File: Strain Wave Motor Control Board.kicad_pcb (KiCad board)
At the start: 2 copper layers, 72 parts, among them J1 GSB1C41110SSHR, J2 S4B-XH-SM4-TB, Q1 CSD18531Q5A, Q2 AO4407A, Q3 CSD18531Q5A, Q4 AO4407A, Q5 SI4178DY-T1-GE3, Q6 AO4407A, U1 HUSB238A-xxxxx-QN16R, U2 BQ7791500PWR, U3 LTC4007, U4 LM2596S-5, U5 ESP32-C6

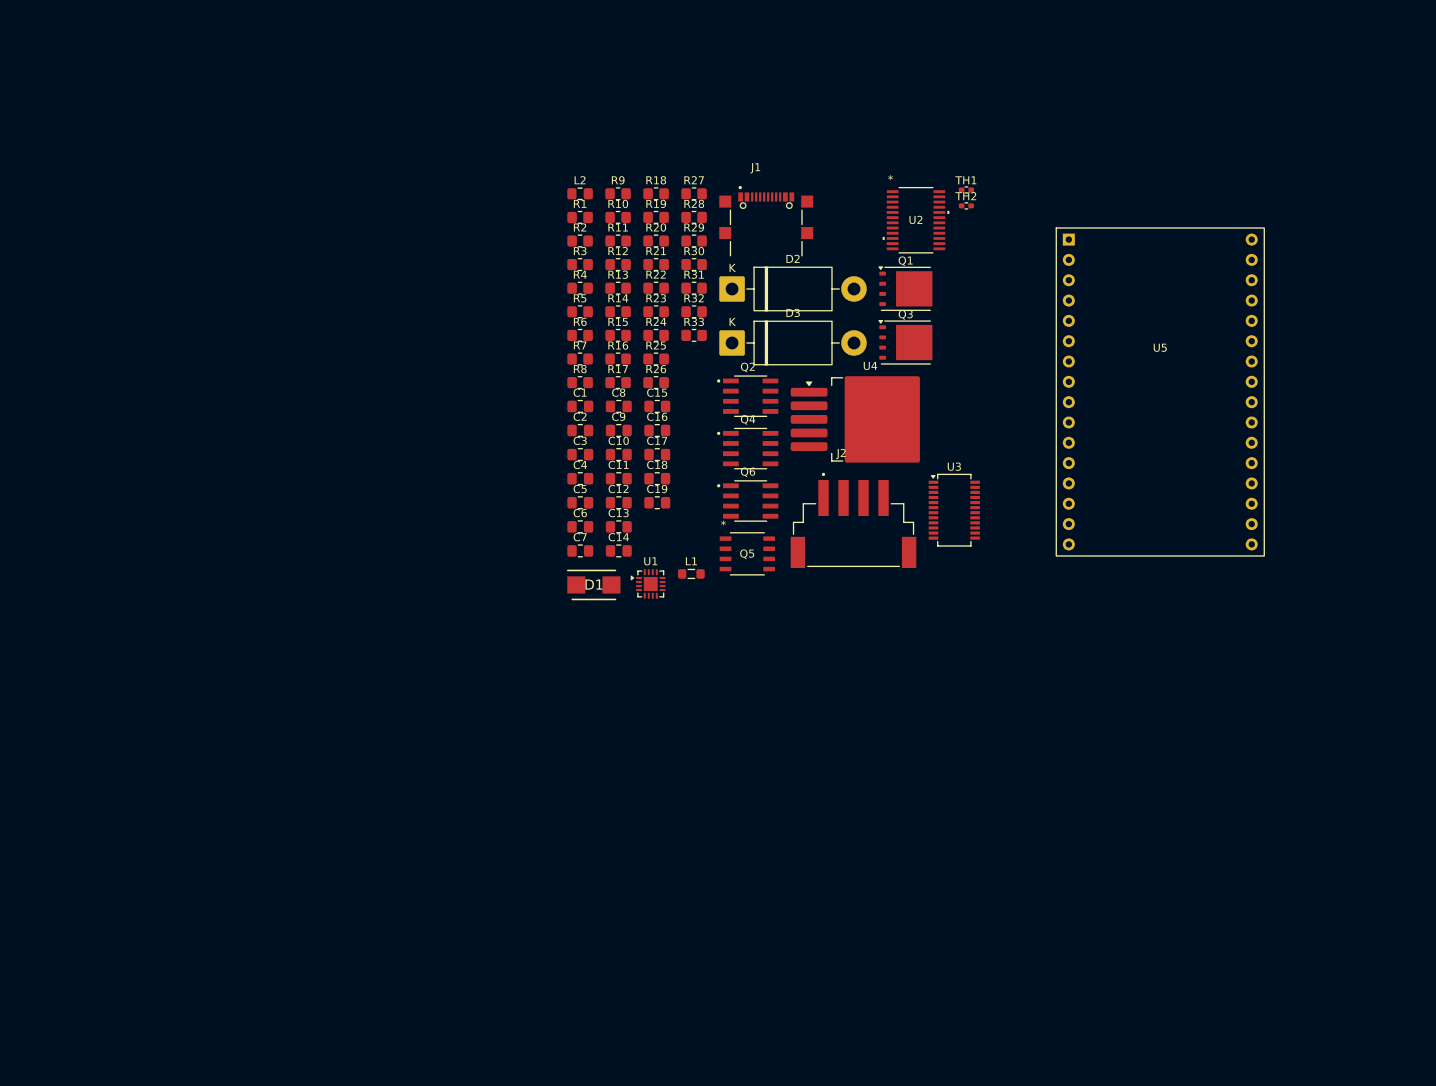
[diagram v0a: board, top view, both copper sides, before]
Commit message: started layout
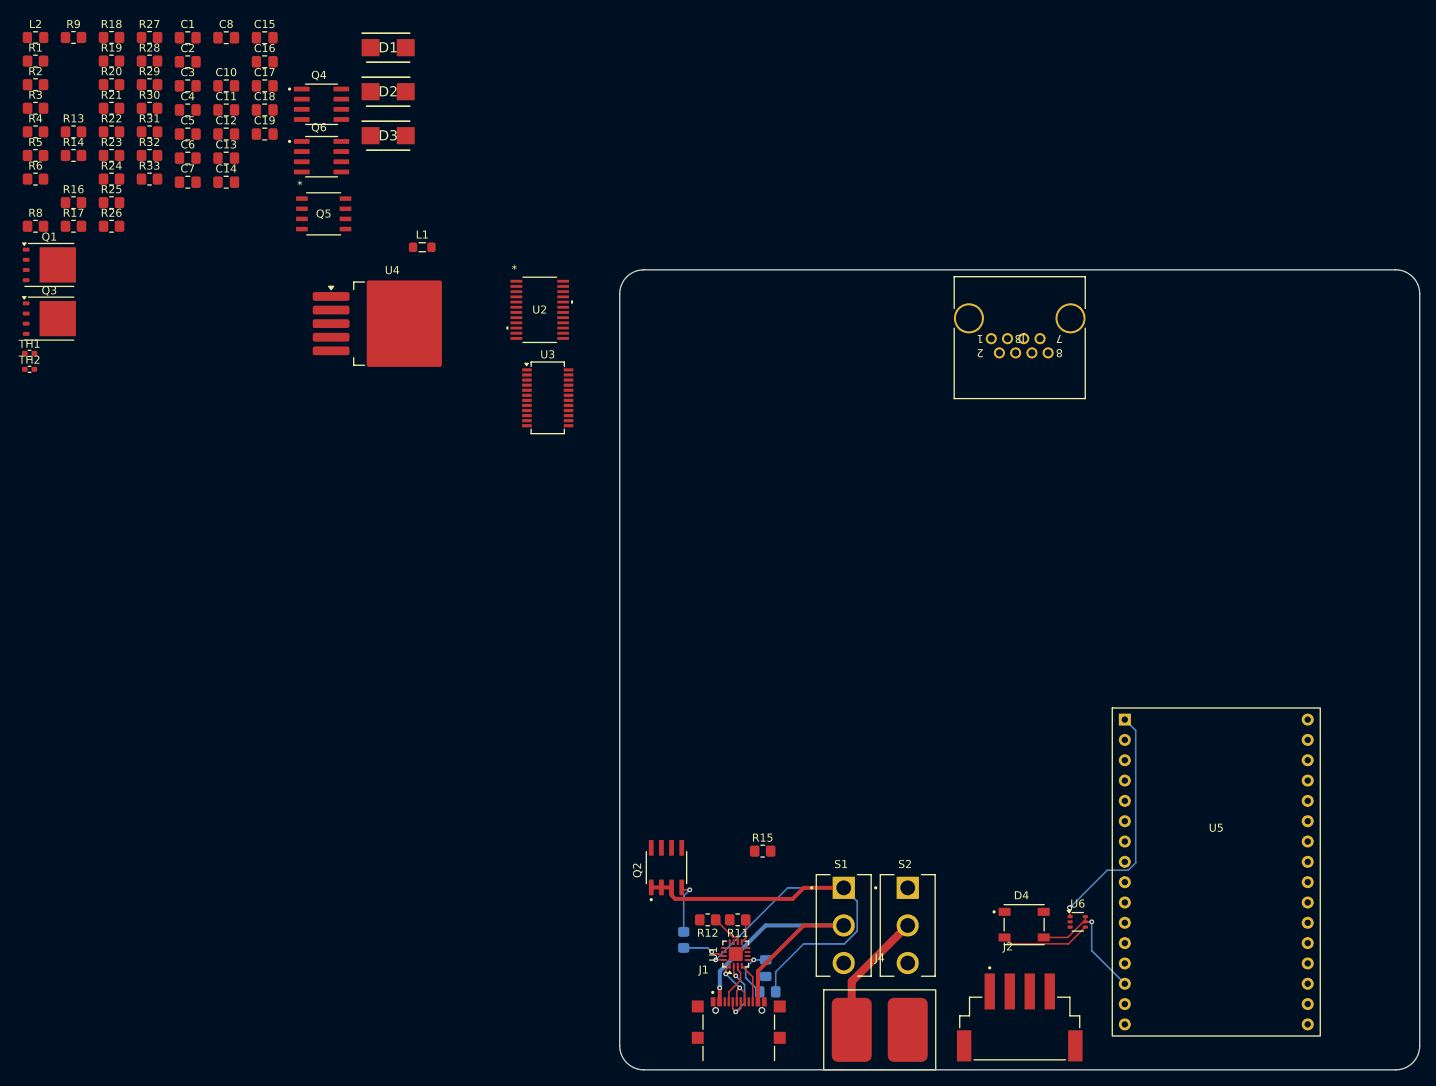
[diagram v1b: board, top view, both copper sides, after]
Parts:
- added D4: 1655, 1655:LED_1655, F.Cu at (150.6, 131.8)
- added J3: RJHSE-5080, RJ45:CONN_RJSBE5080_16P13X12P57_AMP, F.Cu at (146.4, 58.6)
- added J4: ~, Battery_Connector:LiPo Wire Pads, F.Cu at (132.5, 136.5)
- added S1: 100SP1T1B4M2QE, Switches:SW_100SP1T1B4M2QE, F.Cu at (128.0, 131.9)
- added S2: 100SP1T1B4M2QE, Switches:SW_100SP1T1B4M2QE, F.Cu at (136.0, 131.9)
- added U6: SN74LVC1T45DCK, Package_TO_SOT_SMD:SOT-363_SC-70-6, F.Cu at (157.2, 131.5)
- C9, R10, R7: moved to B.Cu
- D2, D3: value 1N5822 -> MBRS130T3G; footprint Diode_THT:D_DO-201AD_P15.24mm_Horizontal -> MBRS130T3G:DIOM5436X247N
- moved TH1 118.9 mm to (26.2, 60.4)
- moved TH2 118.9 mm to (26.2, 62.4)
- moved Q1 107.1 mm to (28.7, 49.4)
- moved Q3 107.1 mm to (28.7, 56.1)
- moved J1 100.7 mm to (114.9, 145.2)
- moved R10 90.7 mm to (108.0, 133.8), turned to 90 degrees
- moved R11 86.2 mm to (114.8, 131.2), turned to 180 degrees
- moved R12 82.7 mm to (111.0, 131.2), turned to 180 degrees
- moved R7 82.5 mm to (118.5, 140.2), turned to 180 degrees
- moved D1 71.9 mm to (71.1, 22.2)
- moved L2 70.8 mm to (27.0, 21.0)
- moved R1 70.8 mm to (27.0, 23.9)
- moved R13 70.8 mm to (31.7, 32.8)
- moved R14 70.8 mm to (31.7, 35.7)
- moved R16 70.8 mm to (31.7, 41.6)
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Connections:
- net /Power Supply/BATT+ renamed /Power Supply/CELL_3
- C19 pad 1: /Power Supply/5V -> /5V
- C5 pad 1: Net-(U2-VDD) -> /Power Supply/PRES
- J1 pad A4_B9: /Power Supply/VBUS -> /Power Supply/USB_VBUS
- J1 pad B4_A9: /Power Supply/VBUS -> /Power Supply/USB_VBUS
- J2 pad 4: /Power Supply/BATT- -> GND
- L2 pad 1: /Power Supply/5V -> /5V
- Q3 pad 1: /Power Supply/BATT- -> /Power Supply/PACK-
- Q3 pad 2: /Power Supply/BATT- -> /Power Supply/PACK-
- Q3 pad 3: /Power Supply/BATT- -> /Power Supply/PACK-
- R1 pad 2: Net-(U2-VDD) -> /Power Supply/PRES
- R17 pad 2: /Power Supply/BATT- -> /Power Supply/PACK-
- R21 pad 2: /Power Supply/BATT- -> /Power Supply/PACK-
- R22 pad 1: /Power Supply/ACP -> /ACP
- R22 pad 2: /Power Supply/VLOGIC -> /VLOGIC
- R23 pad 1: /Power Supply/~FAULT -> /~FAULT
- R23 pad 2: /Power Supply/VLOGIC -> /VLOGIC
- R25 pad 1: /Power Supply/~FLAG -> /~FLAG
- R25 pad 2: /Power Supply/VLOGIC -> /VLOGIC
- U2 pad 1: Net-(U2-VDD) -> /Power Supply/PRES
- U2 pad 16: GND -> unconnected-(U2-CBI-Pad16)
- U2 pad 20: unconnected-(U2-CCFG-Pad20) -> GND
- U2 pad 3: unconnected-(U2-VC5-Pad3) -> Net-(U2-VC3)
- U2 pad 4: unconnected-(U2-VC4-Pad4) -> Net-(U2-VC3)
- U3 pad 13: /Power Supply/~ICL -> /~ICL
- U3 pad 17: /Power Supply/~FLAG -> /~FLAG
- U3 pad 2: /Power Supply/~CHG -> /~CHG
- U3 pad 24: /Power Supply/SHDN -> /SHDN
- U3 pad 3: /Power Supply/ACP -> /ACP
- U3 pad 5: /Power Supply/~FAULT -> /~FAULT
- U3 pad 8: /Power Supply/~LOBAT -> /~LOBAT
- U4 pad 4: /Power Supply/5V -> /5V
- U5 pad 1: unconnected-(U5-3.3V-Pad1) -> /VLOGIC
- U5 pad 10: unconnected-(U5-GPIO10-Pad10) -> /~LOBAT
- U5 pad 11: unconnected-(U5-GPIO11-Pad11) -> /ACP
- U5 pad 12: unconnected-(U5-GPIO2-Pad12) -> /CTRL_1
- U5 pad 13: unconnected-(U5-GPIO3-Pad13) -> /CTRL_2
- U5 pad 14: unconnected-(U5-5V-Pad14) -> /5V
- U5 pad 15: unconnected-(U5-GND-Pad15) -> GND
- U5 pad 17: unconnected-(U5-GND-Pad17) -> GND
- U5 pad 20: unconnected-(U5-GPIO15-Pad20) -> /GPIO_X
- U5 pad 3: unconnected-(U5-GPIO4-Pad3) -> /CTRL_3
- U5 pad 31: unconnected-(U5-GND-Pad31) -> GND
- U5 pad 4: unconnected-(U5-GPIO5-Pad4) -> /SHDN
- U5 pad 5: unconnected-(U5-GPIO6-Pad5) -> /PRES
- U5 pad 6: unconnected-(U5-GPIO7-Pad6) -> /~CHG
- U5 pad 7: unconnected-(U5-GPIO0-Pad7) -> /~FAULT
- U5 pad 8: unconnected-(U5-GPIO1-Pad8) -> /~FLAG
- U5 pad 9: unconnected-(U5-GPIO8-Pad9) -> /~ICL
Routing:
- net /Power Supply/VBUS: track 0.00 -> 67.5 mm, vias 0 -> 1
- net /Power Supply/USB_VBUS: track 0.00 -> 38.6 mm, vias 0 -> 1
- net /VLOGIC: track 0.00 -> 30.2 mm, vias 0 -> 2
- net /5V: track 0.00 -> 16.9 mm, vias 0 -> 1
- net /Power Supply/PACK+: track 0.00 -> 15.9 mm
- net Net-(D4-DIN): track 0.00 -> 11.3 mm
- net /Power Supply/D-: track 0.00 -> 9.81 mm, vias 0 -> 2
- net /Power Supply/D+: track 0.00 -> 7.56 mm, vias 0 -> 2
- net Net-(U1-VDD): track 0.00 -> 7.42 mm, vias 0 -> 1
- net Net-(Q2-Pad4): track 0.00 -> 6.68 mm, vias 0 -> 1
- net Net-(U1-GATE): track 0.00 -> 5.45 mm, vias 0 -> 1
- net /Power Supply/CC1: track 0.00 -> 5.25 mm
- net /Power Supply/CC2: track 0.00 -> 5.07 mm
- net Net-(U1-SCL/SNK_ISET): track 0.00 -> 4.14 mm
- net Net-(U1-SDA/SNK_VSET): track 0.00 -> 3.01 mm
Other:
- board outline added: 100 x 100 mm
